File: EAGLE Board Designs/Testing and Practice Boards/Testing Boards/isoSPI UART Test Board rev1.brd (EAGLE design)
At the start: 160 x 100 mm, 51 parts, among them J1 CONNECTOR-6_μF_T_V_BLACK, J2 CONNECTOR-2_MF_T_V_, J4 CONNECTOR-2_MF_T_V_, J5 CONNECTOR-6_μF_T_V_BLACK, T1 78613/3C, T2 78613/3C, U1 MCP3204, U2 ADM4854ARZ, U3 LTC6820, U4 OPAMP_1_CHANNEL_OPA991, U5 INA823DT, U7 LTC6820

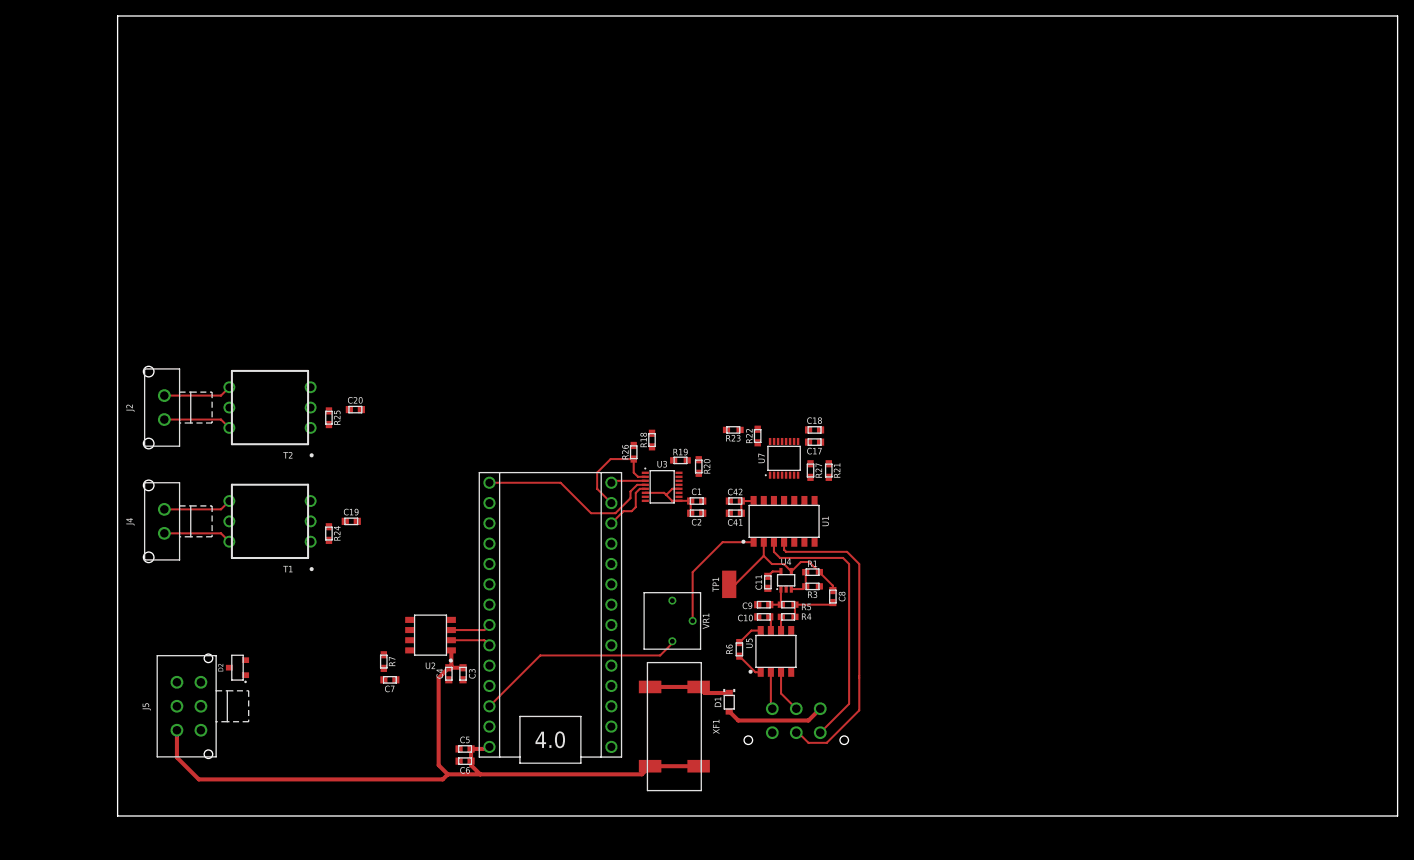
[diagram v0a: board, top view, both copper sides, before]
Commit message: brd rev1 ready for review
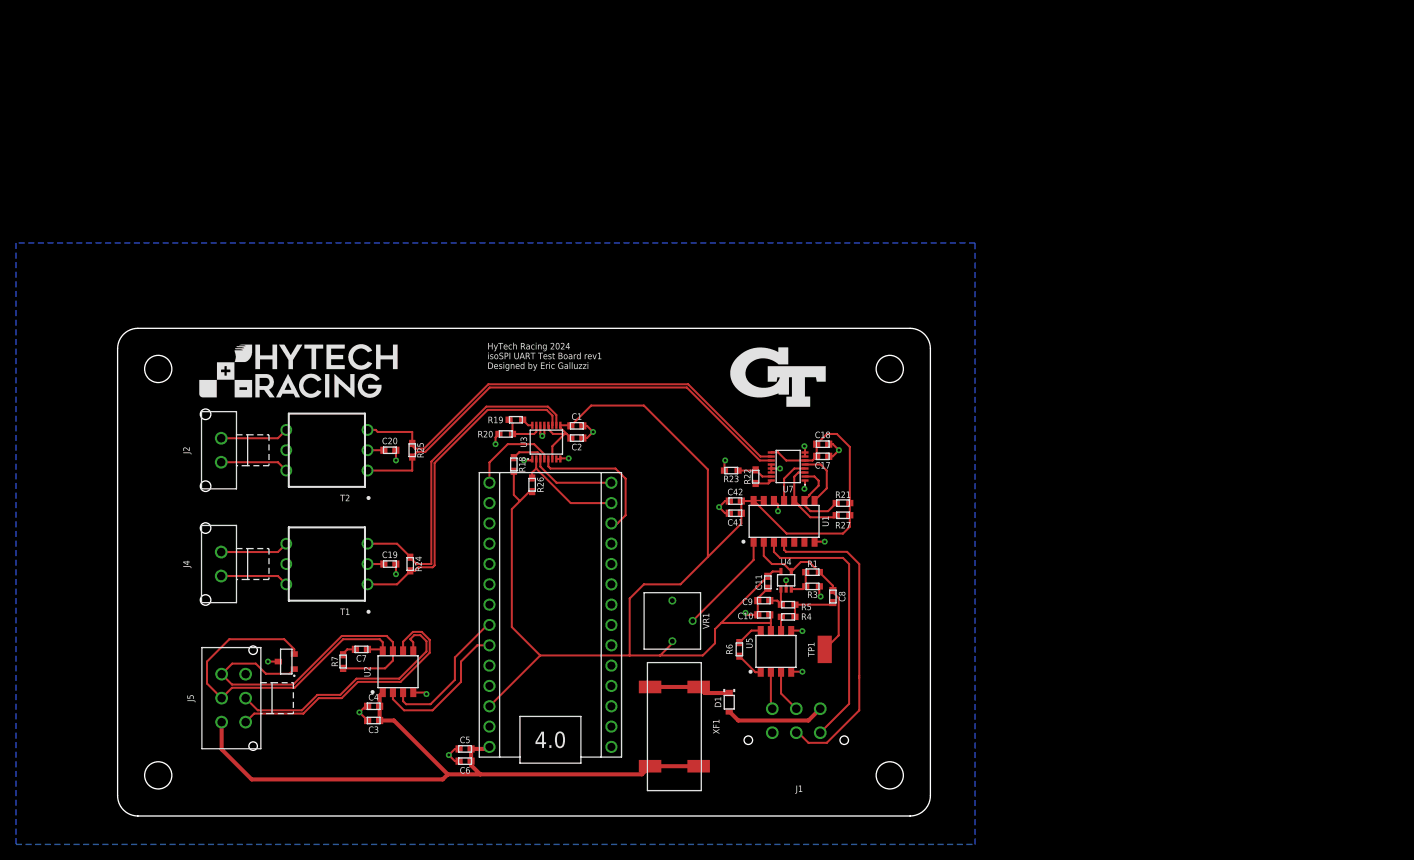
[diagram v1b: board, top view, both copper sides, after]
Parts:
- added U$1, U$2, U$3, U$4: (no value), HyTechManufacturing:MOUNTING_M3
- added U$5: (no value), HyTechManufacturing:LOGO_HYTECH_MEDIUM
- added U$6: (no value), HyTechManufacturing:LOGO_GT_MEDIUM
- moved R20 24.5 mm to (48.5, 47.8), turned to 180 degrees
- moved R19 21.2 mm to (49.8, 49.5), turned to 180 degrees
- moved C1 17.7 mm to (57.4, 48.8)
- moved C2 17.7 mm to (57.4, 47.2)
- moved R18 17.5 mm to (49.5, 43.9), turned to 270 degrees
- moved U3 15.5 mm to (53.6, 46.7), turned to 0 degrees
- moved TP1 14.4 mm to (88.4, 20.8)
- moved R26 13.3 mm to (51.8, 41.4), turned to 270 degrees
- moved C3 12.6 mm to (32.0, 11.9), turned to 180 degrees
- moved R25 11.2 mm to (36.8, 45.7)
- moved R24 10.9 mm to (36.6, 31.5)
- moved C4 10.2 mm to (32.0, 13.7), turned to 180 degrees
- moved J2 8.89 mm to (13.0, 45.7)
- moved J4 8.89 mm to (13.0, 31.5)
- moved T2 8.89 mm to (26.2, 45.7)
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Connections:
- net IP_1 renamed DIFF_1_P
- net IP_2 renamed DIFF_2_P
- net TX+ renamed TX_P
- net TX- renamed TX_N
- removed net IM_1: R24.1, T1.2, U3.10
- removed net IM_2: R25.1, T2.2, U7.10
- removed net RX+: C7.2, D2.1, J5.2, U2.8
- removed net RX-: D2.2, J5.3, R7.1, U2.7
- new net DIFF_1_N: R24.1, T1.3, U3.10
- new net DIFF_2_N: R25.1, T2.3, U7.10
- new net RX_N: D2.1, J5.3, R7.1, U2.7
- new net RX_P: C7.2, D2.2, J5.2, U2.8
- net N$18: now also T1.2; no longer T1.3
- net N$19: now also T2.2; no longer T2.3
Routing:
- net +3V3: track 42.7 -> 192.9 mm
- net DIFF_2_P: track 0.00 -> 59.5 mm
- net DIFF_2_N: track 0.00 -> 59.5 mm
- net GND: track 0.00 -> 47.6 mm, vias 0 -> 24
- net RX_P: track 0.00 -> 44.9 mm
- net RX_N: track 0.00 -> 44.1 mm
- net DIFF_1_N: track 0.00 -> 42.1 mm
- net DIFF_1_P: track 0.00 -> 41.2 mm
- net TX_N: track 0.00 -> 33.6 mm
- net TX_P: track 0.00 -> 31.7 mm
- net UART_RX: track 5.03 -> 18.3 mm
- net UART_TX: track 5.03 -> 17.8 mm
- net TEENSY_CLK: track 23.0 -> 11.5 mm
- net TEENSY_CS: track 7.08 -> 18.0 mm
- net ADC_SDO: track 0.00 -> 10.8 mm
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- added copper zone on layer 16, net GND
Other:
- board size 160 x 100 mm -> 101.6 x 61 mm
- board text added: "HyTech Racing 2024 isoSPI UART Test Board rev1 Designed by Eric Galluzzi"
